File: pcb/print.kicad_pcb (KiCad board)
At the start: 2 copper layers, 0 parts

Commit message: Initial commit
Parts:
- added C1: 100nF, Capacitor_SMD:C_0603_1608Metric, F.Cu at (173.6, 98.3)
- added C10: 100nF, Capacitor_SMD:C_0603_1608Metric, F.Cu at (92.9, 93.6)
- added C2: 1uF, Capacitor_SMD:C_0603_1608Metric, F.Cu at (151.4, 99.9)
- added C3: 1uF, Capacitor_SMD:C_0603_1608Metric, F.Cu at (149.6, 99.9)
- added C4: 4,7uF1 16V, Capacitor_SMD:C_1206_3216Metric, F.Cu at (165.6, 105.0)
- added C5: 100nF, Capacitor_SMD:C_0603_1608Metric, F.Cu at (162.4, 92.0)
- added C6: 100nF, Capacitor_SMD:C_0603_1608Metric, F.Cu at (169.4, 105.3)
- added C7: 100nF, Capacitor_SMD:C_0603_1608Metric, F.Cu at (140.1, 93.6)
- added C8: 100nF, Capacitor_SMD:C_0603_1608Metric, F.Cu at (124.4, 93.6)
- added C9: 100nF, Capacitor_SMD:C_0603_1608Metric, F.Cu at (108.6, 93.6)
- added D1: 5V0, Diode_SMD:D_0603_1608Metric, F.Cu at (175.6, 104.6)
- added D2: 5V0, Diode_SMD:D_0603_1608Metric, F.Cu at (172.6, 104.6)
- added D3: WS2812B, LED_SMD:LED_WS2812B_PLCC4_5.0x5.0mm_P3.2mm, F.Cu at (139.3, 98.1)
- added D4: WS2812B, LED_SMD:LED_WS2812B_PLCC4_5.0x5.0mm_P3.2mm, F.Cu at (123.5, 98.1)
- added D5: WS2812B, LED_SMD:LED_WS2812B_PLCC4_5.0x5.0mm_P3.2mm, F.Cu at (107.8, 98.1)
- added D6: WS2812B, LED_SMD:LED_WS2812B_PLCC4_5.0x5.0mm_P3.2mm, F.Cu at (92.0, 98.1)
- added F1: MFFSMF050, Fuse:Fuse_0603_1608Metric, F.Cu at (173.6, 93.5)
- added J1: USB_leads, Connector_PinHeader_2.54mm:PinHeader_1x04_P2.54mm_Horizontal, F.Cu at (176.5, 94.3)
- added J2: TC2030-IDC-NL, Lib_TC2030-IDC-NL:TC2030-IDC-NL, F.Cu at (153.9, 91.8)
- added R1: 1K0, Resistor_SMD:R_0603_1608Metric, F.Cu at (164.7, 91.3)
- added R2: 1K0, Resistor_SMD:R_0603_1608Metric, F.Cu at (161.4, 94.8)
- added R3: 1K0, Resistor_SMD:R_0603_1608Metric, F.Cu at (160.6, 92.0)
- added R4: 1K0, Resistor_SMD:R_0603_1608Metric, F.Cu at (144.9, 105.2)
- added U1: FT232RL, Package_SO:SSOP-28_5.3x10.2mm_P0.65mm, F.Cu at (168.0, 98.1)
- added U2: ATmega328-A, Package_QFP:TQFP-32_7x7mm_P0.8mm, F.Cu at (157.6, 101.1)
- added Y1: 16MHz, Crystal:Crystal_SMD_3225-4Pin_3.2x2.5mm, F.Cu at (150.0, 103.9)
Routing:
- net +5V: track 0.00 -> 176.3 mm, vias 0 -> 2
- net /RESET: track 0.00 -> 28.9 mm, vias 0 -> 2
- net /SCK: track 0.00 -> 24.8 mm, vias 0 -> 2
- net Net-(D1-A2): track 0.00 -> 24.5 mm
- net /MISO: track 0.00 -> 22.8 mm, vias 0 -> 2
- net /MOSI: track 0.00 -> 20.7 mm, vias 0 -> 2
- net Net-(U2-AREF): track 0.00 -> 19.5 mm, vias 0 -> 2
- net Net-(D3-DOUT): track 0.00 -> 16.5 mm
- net Net-(D4-DOUT): track 0.00 -> 16.5 mm
- net Net-(D5-DOUT): track 0.00 -> 16.4 mm
- net /DATA: track 0.00 -> 13.2 mm
- net GND: track 0.00 -> 10.4 mm, vias 0 -> 132
- net Net-(U2-PD2): track 0.00 -> 10.1 mm
- net Net-(D2-A2): track 0.00 -> 9.76 mm
- net Net-(U2-XTAL2/PB7): track 0.00 -> 7.82 mm
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- added copper zone on B.Cu, net GND
- added copper zone on F.Cu, net GND
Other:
- board outline added: 100 x 22 mm

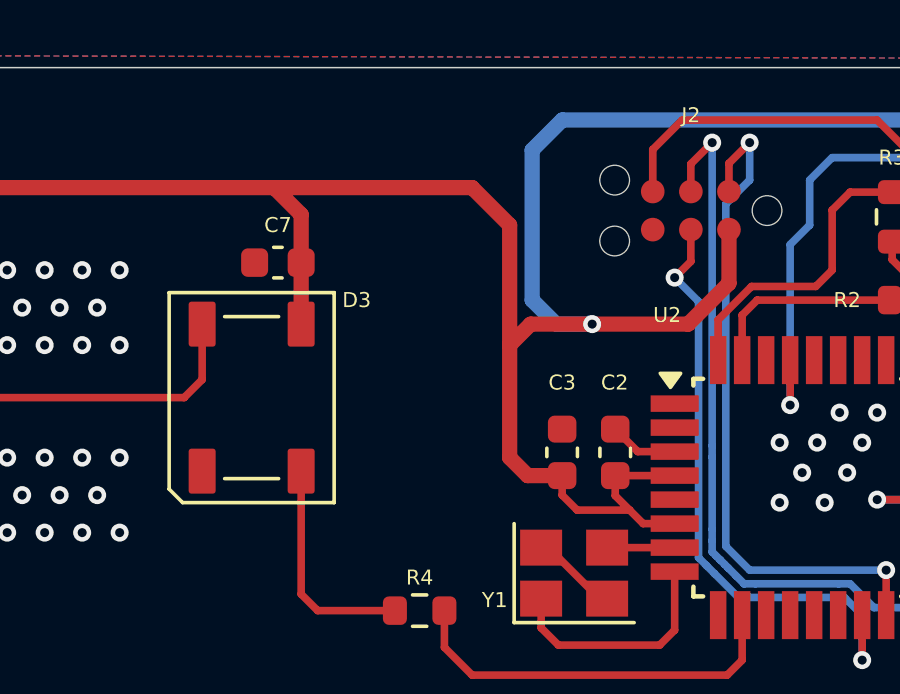
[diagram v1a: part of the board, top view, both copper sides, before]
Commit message: Add files via upload
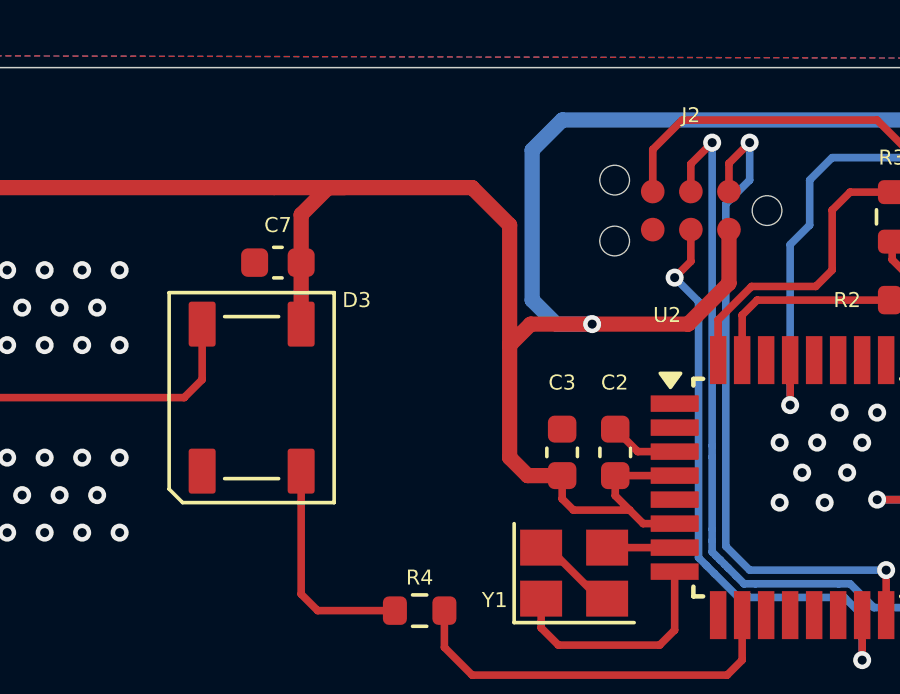
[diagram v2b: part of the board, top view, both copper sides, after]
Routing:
- net +5V: track 176.3 -> 176.9 mm

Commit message: Add files via upload
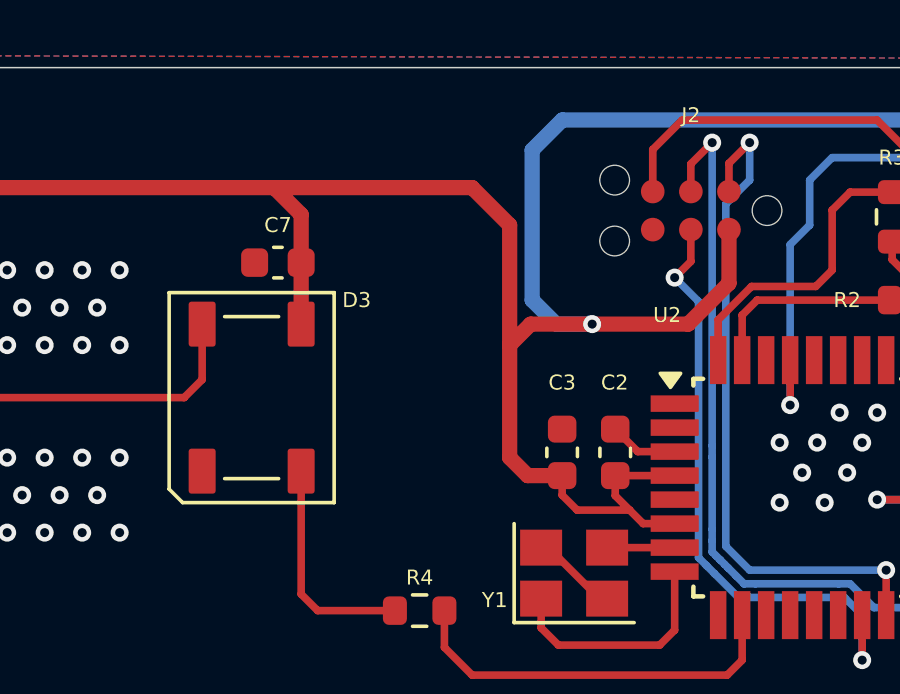
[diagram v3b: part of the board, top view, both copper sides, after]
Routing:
- net +5V: track 176.9 -> 176.3 mm
